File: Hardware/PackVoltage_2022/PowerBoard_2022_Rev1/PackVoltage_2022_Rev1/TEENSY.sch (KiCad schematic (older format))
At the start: 4 parts, among them J1 RJ45_LED_Shielded, U20 Teensy4.1_DEV-16771

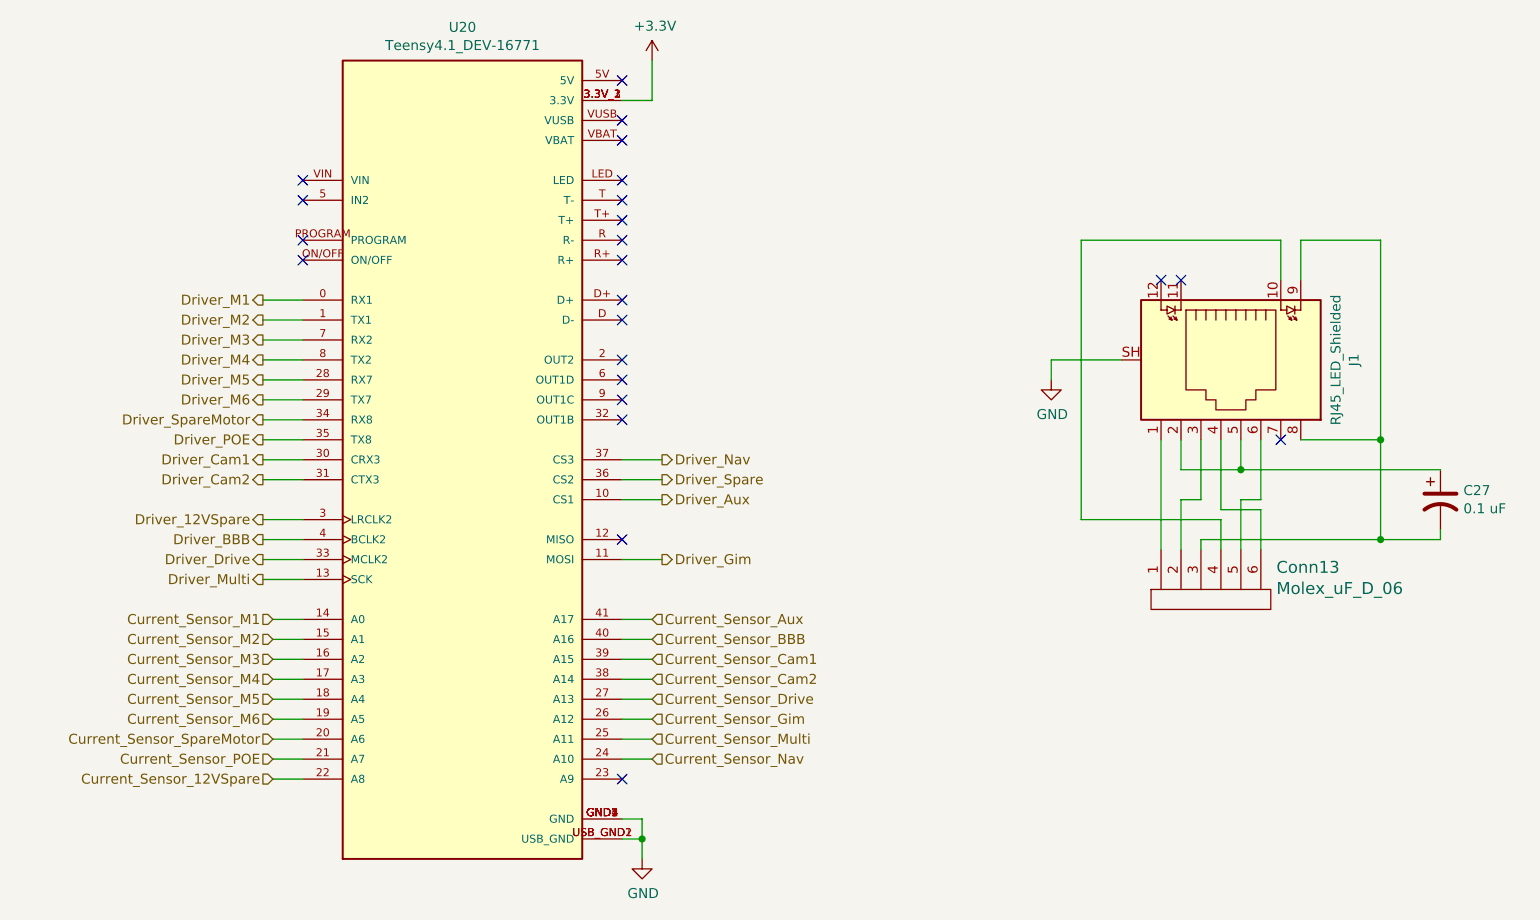
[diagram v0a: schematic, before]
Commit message: All connections made
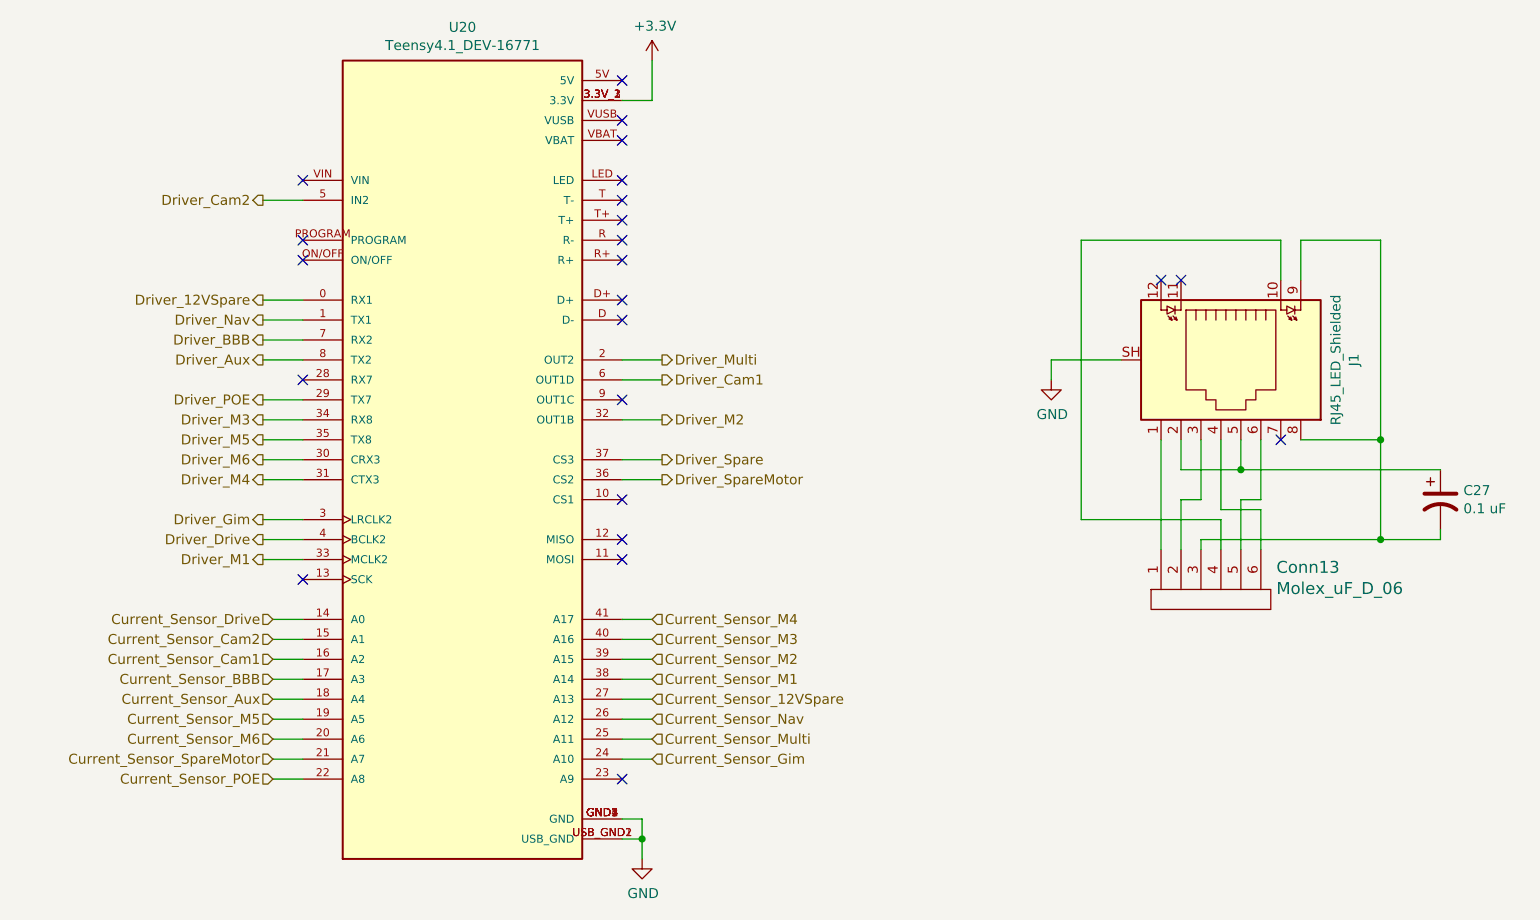
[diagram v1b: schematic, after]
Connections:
- net Current_Sensor_12VSpare: now also U20.27 (A13); no longer U20.22 (A8)
- net Current_Sensor_Aux: now also U20.18 (A4); no longer U20.41 (A17)
- net Current_Sensor_BBB: now also U20.17 (A3); no longer U20.40 (A16)
- net Current_Sensor_Cam1: now also U20.16 (A2); no longer U20.39 (A15)
- net Current_Sensor_Cam2: now also U20.15 (A1); no longer U20.38 (A14)
- net Current_Sensor_Drive: now also U20.14 (A0); no longer U20.27 (A13)
- net Current_Sensor_Gim: now also U20.24 (A10); no longer U20.26 (A12)
- net Current_Sensor_M1: now also U20.38 (A14); no longer U20.14 (A0)
- net Current_Sensor_M2: now also U20.39 (A15); no longer U20.15 (A1)
- net Current_Sensor_M3: now also U20.40 (A16); no longer U20.16 (A2)
- net Current_Sensor_M4: now also U20.41 (A17); no longer U20.17 (A3)
- net Current_Sensor_M5: now also U20.19 (A5); no longer U20.18 (A4)
- net Current_Sensor_M6: now also U20.20 (A6); no longer U20.19 (A5)
- net Current_Sensor_Nav: now also U20.26 (A12); no longer U20.24 (A10)
- net Current_Sensor_POE: now also U20.22 (A8); no longer U20.21 (A7)
- net Current_Sensor_SpareMotor: now also U20.21 (A7); no longer U20.20 (A6)
- net Driver_12VSpare: now also U20.0 (RX1); no longer U20.3 (LRCLK2)
- net Driver_Aux: now also U20.8 (TX2); no longer U20.10 (CS1)
- net Driver_BBB: now also U20.7 (RX2); no longer U20.4 (BCLK2)
- net Driver_Cam1: now also U20.6 (OUT1D); no longer U20.30 (CRX3)
- net Driver_Cam2: now also U20.5 (IN2); no longer U20.31 (CTX3)
- net Driver_Drive: now also U20.4 (BCLK2); no longer U20.33 (MCLK2)
- net Driver_Gim: now also U20.3 (LRCLK2); no longer U20.11 (MOSI)
- net Driver_M1: now also U20.33 (MCLK2); no longer U20.0 (RX1)
- net Driver_M2: now also U20.32 (OUT1B); no longer U20.1 (TX1)
- net Driver_M3: now also U20.34 (RX8); no longer U20.7 (RX2)
- net Driver_M4: now also U20.31 (CTX3); no longer U20.8 (TX2)
- net Driver_M5: now also U20.35 (TX8); no longer U20.28 (RX7)
- net Driver_M6: now also U20.30 (CRX3); no longer U20.29 (TX7)
- net Driver_Multi: now also U20.2 (OUT2); no longer U20.13 (SCK)
- net Driver_Nav: now also U20.1 (TX1); no longer U20.37 (CS3)
- net Driver_POE: now also U20.29 (TX7); no longer U20.35 (TX8)
- net Driver_Spare: now also U20.37 (CS3); no longer U20.36 (CS2)
- net Driver_SpareMotor: now also U20.36 (CS2); no longer U20.34 (RX8)
